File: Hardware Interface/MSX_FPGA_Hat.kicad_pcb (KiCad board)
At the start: 2 copper layers, 99.9 x 64 mm, 37 parts, among them J1 J1, J2 J2, J5 Conn_01x03_Female, Q1 2N3904, Q2 2N3904, SW1 SW_Push, U1 74LVC245, U2 74LVC245, U3 74LVC245, U4 74LVC245, U5 74LVC245, U6 LM1117-3.3

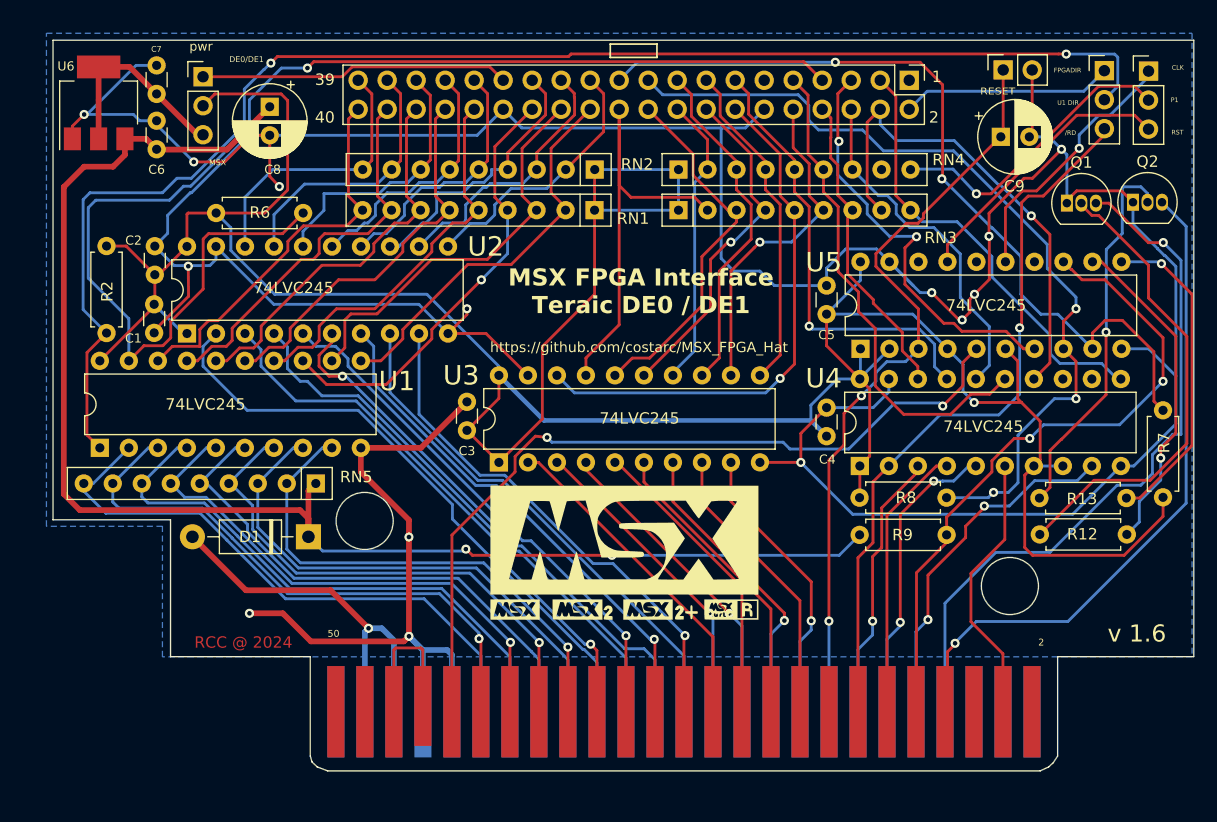
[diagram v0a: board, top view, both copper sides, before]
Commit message: Version 2.0
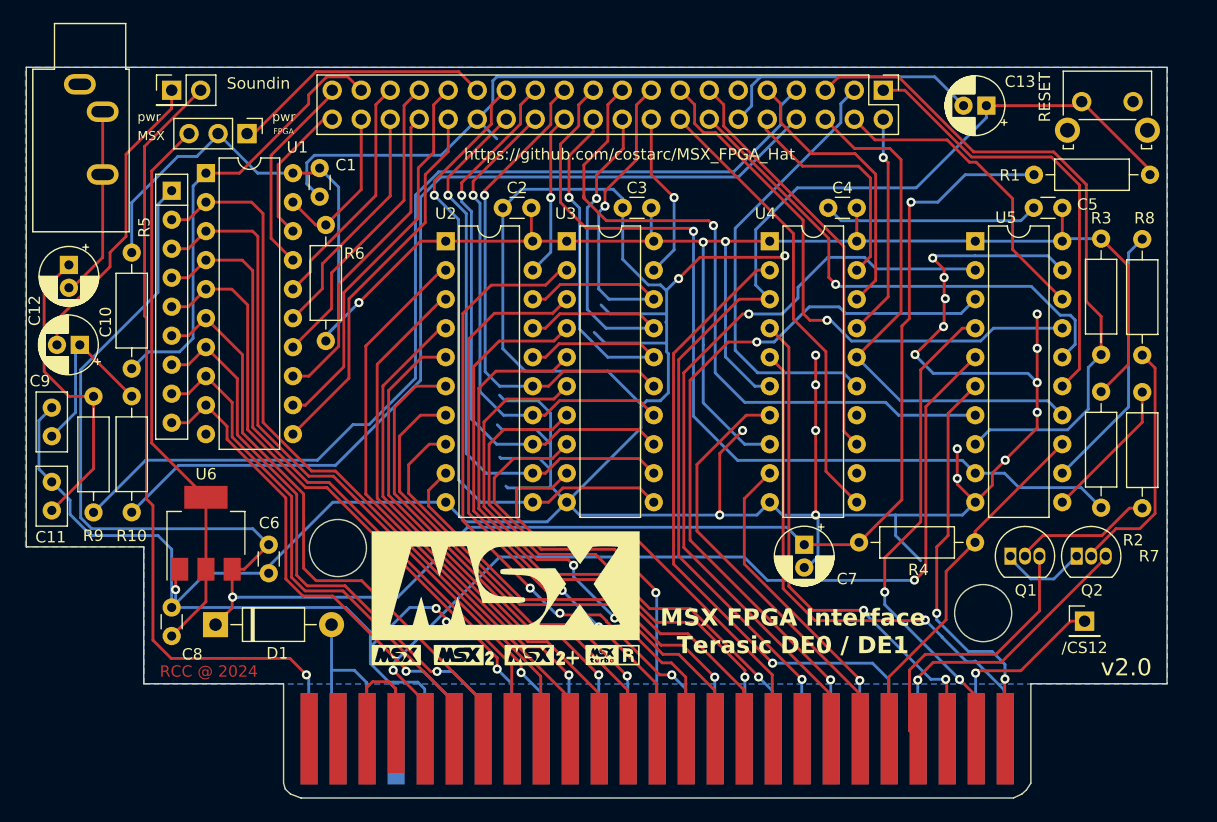
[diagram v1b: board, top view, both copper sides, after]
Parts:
- removed J5: Conn_01x03_Female, Connector_PinHeader_2.54mm:PinHeader_1x03_P2.54mm_Vertical
- removed R12, R13: 2K2, Resistor_THT:R_Axial_DIN0207_L6.3mm_D2.5mm_P7.62mm_Horizontal
- removed RN2, RN3, RN4, RN5: 10K, Resistor_THT:R_Array_SIP9
- added C10: 10uF, Capacitor_THT:CP_Radial_D5.0mm_P2.00mm, F.Cu at (55.0, 48.9)
- added C11: 105, Capacitor_THT:C_Disc_D5.0mm_W2.5mm_P2.50mm, F.Cu at (52.5, 63.4)
- added C12: 10uF, Capacitor_THT:CP_Radial_D5.0mm_P2.00mm, F.Cu at (54.0, 41.9)
- added C13: 100uF, Capacitor_THT:CP_Radial_D5.0mm_P2.00mm, F.Cu at (134.4, 27.9)
- added J3: AudioJack3, Connector_Audio:Jack_3.5mm_CUI_SJ1-3533NG_Horizontal, F.Cu at (55.0, 26.1)
- added J4: /CS12, Connector_PinHeader_2.54mm:PinHeader_1x01_P2.54mm_Vertical, F.Cu at (143.0, 73.1)
- added R1: 10K, Resistor_THT:R_Axial_DIN0207_L6.3mm_D2.5mm_P10.16mm_Horizontal, F.Cu at (138.6, 34.0)
- added R10: 47, Resistor_THT:R_Axial_DIN0207_L6.3mm_D2.5mm_P10.16mm_Horizontal, F.Cu at (59.5, 63.5)
- added R3: 4K7, Resistor_THT:R_Axial_DIN0207_L6.3mm_D2.5mm_P10.16mm_Horizontal, F.Cu at (144.4, 39.6)
- added R4: 10K, Resistor_THT:R_Axial_DIN0207_L6.3mm_D2.5mm_P10.16mm_Horizontal, F.Cu at (123.2, 66.2)
- added R5: 10K, Resistor_THT:R_Axial_DIN0207_L6.3mm_D2.5mm_P10.16mm_Horizontal, F.Cu at (59.5, 40.8)
- C7: value 0.1uf -> 10uF; footprint Capacitor_THT:C_Disc_D3.0mm_W1.6mm_P2.50mm -> Capacitor_THT:CP_Radial_D5.0mm_P2.00mm
- C8: value 10uF -> 0.1uf; footprint Capacitor_THT:CP_Radial_D6.3mm_P2.50mm -> Capacitor_THT:C_Disc_D3.0mm_W1.6mm_P2.50mm
- C9: value 100uF -> 105; footprint Capacitor_THT:CP_Radial_D6.3mm_P2.50mm -> Capacitor_THT:C_Disc_D5.0mm_W2.5mm_P2.50mm
- J1: value J1 -> Conn_01x03_Female
- J2: value J2 -> Soundin; footprint Connector_PinHeader_2.54mm:PinHeader_1x03_P2.54mm_Vertical -> Connector_PinHeader_2.54mm:PinHeader_2x01_P2.54mm_Vertical
- R2: value 10K -> 4K7; footprint Resistor_THT:R_Axial_DIN0207_L6.3mm_D2.5mm_P7.62mm_Horizontal -> Resistor_THT:R_Axial_DIN0207_L6.3mm_D2.5mm_P10.16mm_Horizontal
- R6: footprint Resistor_THT:R_Axial_DIN0207_L6.3mm_D2.5mm_P7.62mm_Horizontal -> Resistor_THT:R_Axial_DIN0207_L6.3mm_D2.5mm_P10.16mm_Horizontal
- R7, R8: value 4K7 -> 2K2; footprint Resistor_THT:R_Axial_DIN0207_L6.3mm_D2.5mm_P7.62mm_Horizontal -> Resistor_THT:R_Axial_DIN0207_L6.3mm_D2.5mm_P10.16mm_Horizontal
- R9: value 10K -> 47; footprint Resistor_THT:R_Axial_DIN0207_L6.3mm_D2.5mm_P7.62mm_Horizontal -> Resistor_THT:R_Axial_DIN0207_L6.3mm_D2.5mm_P10.16mm_Horizontal
- SW1: value SW_Push -> RESET; footprint Connector_PinSocket_2.54mm:PinSocket_1x02_P2.54mm_Vertical -> Button_Switch_THT:SW_Tactile_SKHH_Angled
- moved R2 88.0 mm to (144.4, 53.0)
- moved C9 87.2 mm to (52.5, 56.9), turned to 90 degrees
- moved J2 85.6 mm to (63.0, 26.6)
- moved J1 75.3 mm to (69.6, 30.4), turned to -90 degrees
- moved C7 69.1 mm to (118.4, 66.4), turned to -90 degrees
- moved R9 67.1 mm to (56.2, 63.6), turned to 90 degrees
- moved C8 47.1 mm to (63.0, 74.4), turned to 90 degrees
- moved U6 38.8 mm to (66.0, 65.4)
- moved RN1 37.1 mm to (63.0, 35.4), turned to -90 degrees
- moved C6 36.0 mm to (71.5, 66.4), turned to -90 degrees
- moved C2 33.5 mm to (94.5, 36.9), turned to 180 degrees
- moved Q2 31.4 mm to (142.3, 67.4)
- moved Q1 31.3 mm to (136.5, 67.4)
- moved R8 27.7 mm to (148.0, 49.8), turned to 90 degrees
- moved U1 25.8 mm to (66.0, 33.8), turned to 0 degrees
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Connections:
- C7 pad 1: MSX_3.3V -> Vcc
- C8 pad 1: Vcc -> MSX_3.3V
- C9 pad 1: /RESET -> Net-(C10-Pad1)
- CONN1 pad 1: unconnected-(CONN1-/CS1-Pad1) -> /CS1
- CONN1 pad 2: unconnected-(CONN1-/CS2-Pad2) -> /CS2
- CONN1 pad 3: unconnected-(CONN1-/CS12-Pad3) -> /CS12
- CONN1 pad 49: unconnected-(CONN1-SOUNDIN-Pad49) -> SOUNDIN
- CONN1 pad 6: unconnected-(CONN1-/RFSH-Pad6) -> /RFSH
- IDC1 pad 1: C_RST -> C_CLOCK
- IDC1 pad 10: C_A15 -> /C_U4_OE
- IDC1 pad 11: DE_5V -> unconnected-(IDC1-Pin_11-Pad11)
- IDC1 pad 13: /C_WR -> /C_MREQ
- IDC1 pad 14: C_A8 -> /C_SLTSL
- IDC1 pad 15: C_A9 -> /C_WR
- IDC1 pad 16: C_A6 -> /C_IORQ
- IDC1 pad 17: C_A11 -> A4_12
- IDC1 pad 18: C_A10 -> /C_U3_OE
- IDC1 pad 19: /C_WAIT -> /C_BUSDIR
- IDC1 pad 2: C_DATA_DIR -> /C_RESET
- IDC1 pad 20: C_A7 -> A5_13
- IDC1 pad 22: C_A12 -> A2_10
- IDC1 pad 23: C_A13 -> A3_11
- IDC1 pad 24: C_D0 -> /C_U2_OE
- IDC1 pad 25: C_A14 -> A1_9
- IDC1 pad 26: C_D1 -> A0_8
- IDC1 pad 27: C_A0 -> A7_15
- IDC1 pad 28: C_D2 -> A6_14
- IDC1 pad 3: /C_M1 -> /C_CS1
- IDC1 pad 31: C_A1 -> C_D6
- IDC1 pad 32: C_D3 -> C_D7
- IDC1 pad 33: C_A2 -> C_D4
- IDC1 pad 34: C_D4 -> C_D5
- IDC1 pad 35: C_A3 -> C_D2
- IDC1 pad 36: C_D5 -> C_D3
- IDC1 pad 37: C_A4 -> /U1_D_DIR
- IDC1 pad 38: C_D6 -> /C_U1_OE
- IDC1 pad 39: C_A5 -> C_D1
- IDC1 pad 4: /C_SLTSL -> /C_RD
- IDC1 pad 40: C_D7 -> C_D0
- IDC1 pad 5: /C_BUSDIR -> /C_WAIT
- IDC1 pad 6: /C_MREQ -> /C_CS2_RFSH
- IDC1 pad 7: /C_U1_D_OE -> C_SOUND
- IDC1 pad 8: /C_RD -> C_AUDIO
- IDC1 pad 9: /C_IORQ -> /C_M1
- J1 pad 1: C_DATA_DIR -> DE_3.3V
- J1 pad 2: /U1_D_DIR -> Vdd
- J1 pad 3: /RD -> MSX_3.3V
- J2 pad 1: C_CLOCK -> Net-(J2-Pin_1)
- J2 pad 2: C_CLK_OR_RST -> SOUNDIN
- Q1 pad 3: /WAIT -> /INT
- Q2 pad 3: /INT -> /WAIT
- R2 pad 2: /U1_D_DIR -> /C_INT
- R6 pad 2: /C_U1_D_OE -> /C_U1_OE
- R7 pad 1: Vdd -> Net-(Q1-B)
- R7 pad 2: /C_INT -> Net-(U5-B8)
- R8 pad 1: Vdd -> Net-(Q2-B)
- R8 pad 2: /C_WAIT -> Net-(U5-B7)
- R9 pad 1: Vcc -> C_SOUND
- R9 pad 2: /BUSDIR -> Net-(C11-Pad1)
- RN1 pad 1: Vdd -> Vcc
- RN1 pad 2: C_D0 -> D0
- RN1 pad 3: C_D1 -> D1
- RN1 pad 4: C_D2 -> D2
- RN1 pad 5: C_D3 -> D3
- RN1 pad 6: C_D4 -> D4
- RN1 pad 7: C_D5 -> D5
- RN1 pad 8: C_D6 -> D6
- RN1 pad 9: C_D7 -> D7
- U1 pad 11: C_D0 -> C_D7
- U1 pad 12: C_D1 -> C_D6
- U1 pad 13: C_D2 -> C_D5
- U1 pad 14: C_D3 -> C_D4
- U1 pad 15: C_D4 -> C_D3
- U1 pad 16: C_D5 -> C_D2
- U1 pad 17: C_D6 -> C_D1
- U1 pad 18: C_D7 -> C_D0
- U1 pad 19: /C_U1_D_OE -> /C_U1_OE
- U1 pad 2: D7 -> D0
- U1 pad 3: D6 -> D1
- U1 pad 4: D5 -> D2
- U1 pad 5: D4 -> D3
- U1 pad 6: D3 -> D4
- U1 pad 7: D2 -> D5
- U1 pad 8: D1 -> D6
- U1 pad 9: D0 -> D7
- U2 pad 11: C_A13 -> A7_15
- U2 pad 12: C_A14 -> A6_14
- U2 pad 13: C_A0 -> A1_9
- U2 pad 14: C_A1 -> A0_8
- U2 pad 15: C_A2 -> A3_11
- U2 pad 16: C_A3 -> A2_10
- U2 pad 17: C_A4 -> A5_13
- U2 pad 18: C_A5 -> A4_12
- U2 pad 19: GNDREF -> /C_U2_OE
- U2 pad 2: A5 -> A4
- U2 pad 3: A4 -> A5
- U2 pad 4: A3 -> A2
- U2 pad 5: A2 -> A3
- U2 pad 6: A1 -> A0
- U2 pad 7: A0 -> A1
- U2 pad 8: A14 -> A6
- U2 pad 9: A13 -> A7
- U3 pad 11: C_A9 -> A7_15
- U3 pad 12: C_A15 -> A6_14
- U3 pad 13: C_A11 -> A1_9
- U3 pad 14: C_A10 -> A0_8
- U3 pad 15: C_A6 -> A3_11
- U3 pad 16: C_A7 -> A2_10
- U3 pad 17: C_A12 -> A5_13
- U3 pad 18: C_A8 -> A4_12
- U3 pad 19: GNDREF -> /C_U3_OE
- U3 pad 2: A8 -> A12
- U3 pad 3: A12 -> A13
- U3 pad 4: A7 -> A10
- U3 pad 5: A6 -> A11
- U3 pad 6: A10 -> A8
- U3 pad 7: A11 -> A9
- U3 pad 8: A15 -> A14
- U3 pad 9: A9 -> A15
- U4 pad 11: /C_M1 -> /C_IORQ
- U4 pad 12: /C_CS2 -> unconnected-(U4-B7-Pad12)
- U4 pad 13: /C_CS1 -> /C_MREQ
- U4 pad 14: /C_SLTSL -> unconnected-(U4-B5-Pad14)
- U4 pad 15: /C_IORQ -> /C_CS1
- U4 pad 16: /C_MREQ -> /C_CS2_RFSH
- U4 pad 17: /C_WR -> /C_RESET
- U4 pad 18: /C_RD -> /C_M1
- U4 pad 19: GNDREF -> /C_U4_OE
- U4 pad 2: /RD -> /M1
- U4 pad 3: /WR -> /RESET
- U4 pad 4: /MREQ -> /RFSH
- U4 pad 5: /IORQ -> /CS1
- U4 pad 6: /SLTSL -> Vdd
- U4 pad 7: Vdd -> /MREQ
- U4 pad 9: /M1 -> /IORQ
- U5 pad 14: unconnected-(U5-B5-Pad14) -> /C_CS2_RFSH
- U5 pad 16: unconnected-(U5-B3-Pad16) -> /C_SLTSL
- U5 pad 17: /C_RESET -> /C_WR
- U5 pad 18: unconnected-(U5-B1-Pad18) -> /C_RD
- U5 pad 2: Vdd -> /RD
- U5 pad 3: /RESET -> /WR
- U5 pad 4: Vdd -> /SLTSL
- U5 pad 6: Vdd -> /CS2
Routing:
- net /C_U1_D_OE: track 110.6 -> 0.00 mm, vias 1 -> 0
- net GNDREF: track 369.6 -> 468.0 mm, vias 14 -> 23
- net Vdd: track 268.0 -> 178.1 mm, vias 1 -> 3
- net C_SOUND: track 0.00 -> 87.2 mm
- net /U1_D_DIR: track 126.2 -> 39.5 mm, vias 2 -> 0
- net C_AUDIO: track 0.00 -> 81.8 mm
- net SOUNDIN: track 0.00 -> 70.9 mm, vias 0 -> 1
- net A7_15: track 0.00 -> 56.6 mm, vias 0 -> 1
- net A6_14: track 0.00 -> 50.7 mm, vias 0 -> 1
- net A1_9: track 0.00 -> 49.8 mm, vias 0 -> 1
- net /CS1: track 0.00 -> 48.2 mm, vias 0 -> 1
- net /C_CS2_RFSH: track 0.00 -> 47.8 mm
- net C_A8: track 47.0 -> 0.00 mm, vias 1 -> 0
- net /RFSH: track 0.00 -> 45.3 mm, vias 0 -> 2
- net A3_11: track 0.00 -> 44.0 mm, vias 0 -> 1
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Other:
- board text added: "FPGA"
- board text added: "MSX FPGA Interface Terasic DE0 / DE1"
- board text added: "v2.0"
- board text removed: "/RD"
- board text removed: "1"
- board text removed: "2"
- board text removed: "39"
- board text removed: "40"
- board text removed: "49"
- board text removed: "50"
- board text removed: "CLK"
- board text removed: "DE0/DE1"
- board text removed: "FPGADIR"
- board text removed: "MSX FPGA Interface Teraic DE0 / DE1"
- board text removed: "P1"
- board text removed: "RESET"
- board text removed: "RST"
- board text removed: "U1 DIR"
- board text removed: "v 1.6"
